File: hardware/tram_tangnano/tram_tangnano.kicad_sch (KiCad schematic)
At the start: 61 parts, among them J1 Conn_01x01_SolderingPad, J10 Conn_01x01_SolderingPad, J11 Conn_01x01_SolderingPad, J12 Conn_01x01_SolderingPad, J13 Conn_01x01_SolderingPad, J14 Conn_01x01_SolderingPad, J15 Conn_01x01_SolderingPad, J16 Conn_01x01_SolderingPad, J17 Conn_01x01_SolderingPad, J18 Conn_01x01_SolderingPad, J19 Conn_01x01_SolderingPad, J2 Conn_01x01_SolderingPad, J20 Conn_01x01_SolderingPad, J21 Conn_01x01_SolderingPad, J22 Conn_01x01_SolderingPad, J23 Conn_01x01_SolderingPad, J24 Conn_01x01_SolderingPad, J3 Conn_01x04_Voltage, J4 Conn_01x01_SolderingPad, J5 Conn_01x01_SolderingPad, J6 Conn_01x01_SolderingPad, J7 Conn_01x01_SolderingPad, J8 Conn_01x01_SolderingPad, J9 Conn_01x01_SolderingPad, U1 Tang_Nano_20K, U10 TXU0202, U11 TXU0202, U12 TXU0202, U13 TXU0202, U20 TRAM, U4 SN74LVC2GU04, U6 SN74LVC1G06, U7 SN74LVC1G04

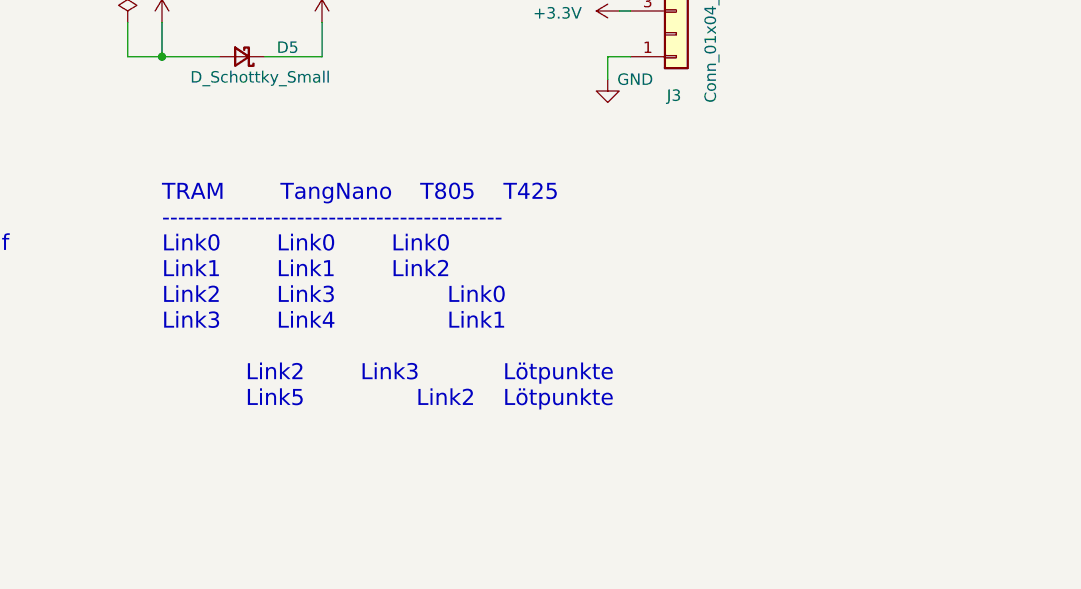
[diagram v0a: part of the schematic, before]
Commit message: Change to 10.x
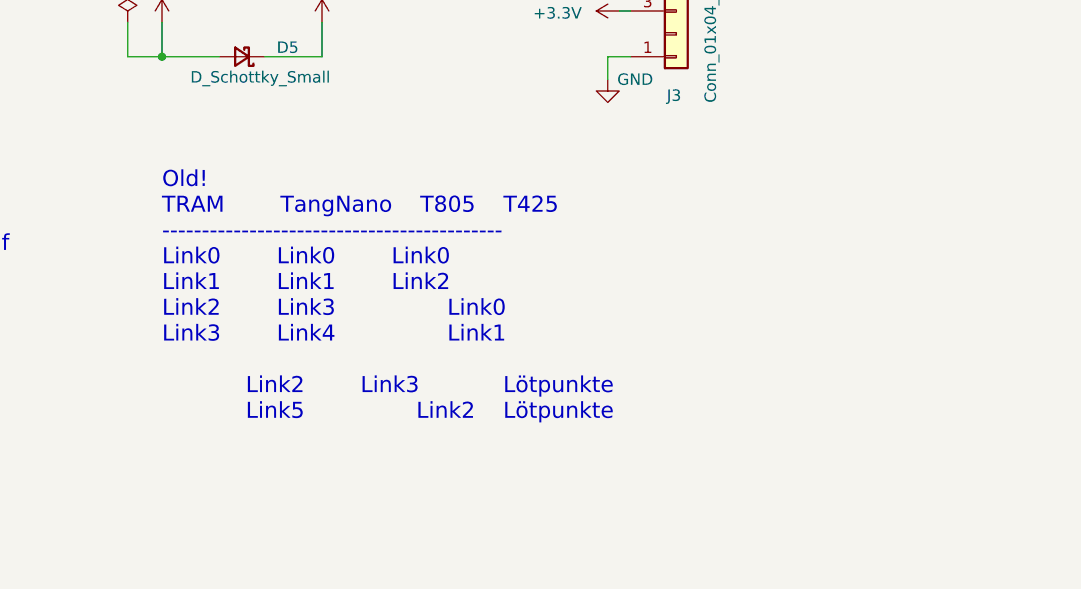
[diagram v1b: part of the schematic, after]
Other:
- note added: "Old! TRAM TangNano T805 T425 ------------------------------------------- Link0 Link0 Link0 Link1 Link1 Link2 Link2 Link3 Link0 Link3 Link4 Link1 Link2 Link3 Lötpunkte Link5 Link2 Lötpunkte"
- note removed: "TRAM TangNano T805 T425 ------------------------------------------- Link0 Link0 Link0 Link1 Link1 Link2 Link2 Link3 Link0 Link3 Link4 Link1 Link2 Link3 Lötpunkte Link5 Link2 Lötpunkte"
